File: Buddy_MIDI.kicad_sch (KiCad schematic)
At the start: 20 parts, among them J1 AudioJack3, J2 AudioJack3, J3 Conn_01x04_Socket, Q2 2N2222, U1 4N25, U2 SN74LVC1G14DBV

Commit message: Remove header from BOM
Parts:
- J3: now left out of the parts list
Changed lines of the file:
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@@
 		(unit 1)
 		(exclude_from_sim no)
-		(in_bom yes)
+		(in_bom no)
 		(on_board yes)
 		(dnp no)
@@
 			(at 97.79 64.77 0)
 			(effects
+				(font
+					(size 1.27 1.27)
+				)
+				(hide yes)
+			)
+		)
+		(property "LCSC Part #" ""
+			(at 97.79 64.77 0)
+			(effects
+				(font
+					(size 1.27 1.27)
+				)
+				(hide yes)
+			)
+		)
+		(property "Part #" ""
+			(at 97.79 64.77 0)
+			(effects

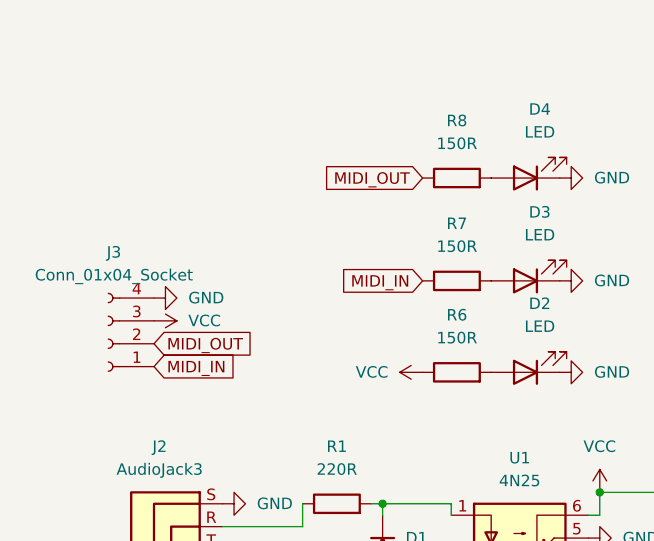
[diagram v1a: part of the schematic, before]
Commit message: New form factor
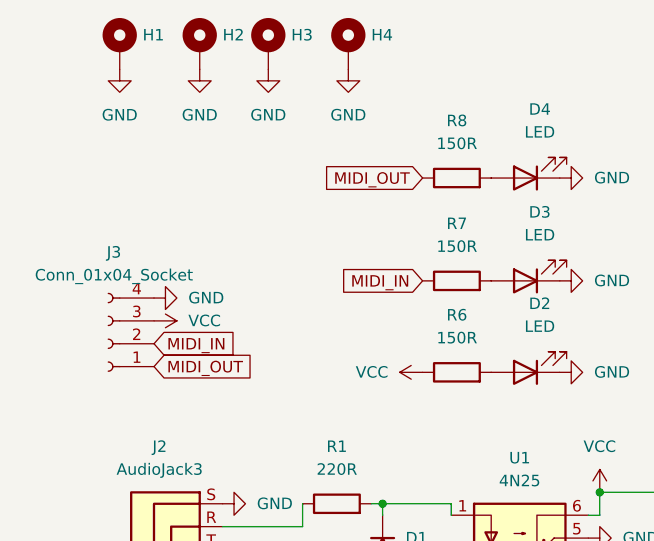
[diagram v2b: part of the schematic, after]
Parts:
- added H1, H2, H3, H4: MountingHole_Pad, MountingHole:MountingHole_2.2mm_M2_Pad, symbol Mechanical:MountingHole_Pad
- J1, J2: footprint Connector_Audio:Jack_3.5mm_CUI_SJ1-3523N_Horizontal -> Connector_Audio:Jack_3.5mm_QingPu_WQP-PJ398SM_Vertical_CircularHoles
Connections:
- net GND: now also H1.1, H2.1, H3.1, H4.1
- net MIDI_IN: now also J3.2 (Pin_2); no longer J3.1 (Pin_1)
- net MIDI_OUT: now also J3.1 (Pin_1); no longer J3.2 (Pin_2)
